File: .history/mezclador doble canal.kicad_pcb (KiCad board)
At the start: 2 copper layers, 166 x 100.5 mm, 17 parts, among them J1 Conn_Coaxial, J2 Conn_Coaxial, J3 Conn_Coaxial, U1 NE5532

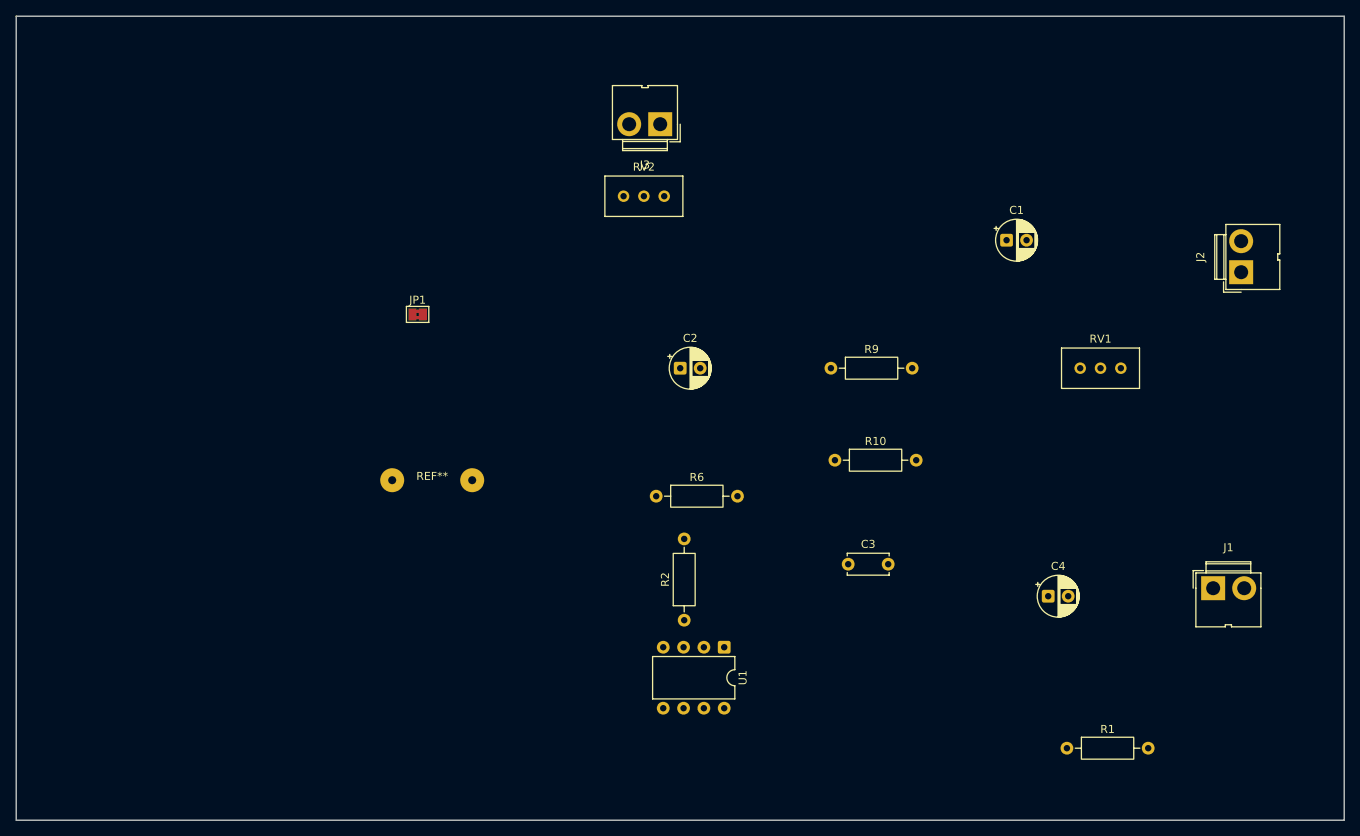
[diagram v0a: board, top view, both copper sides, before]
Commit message: completè el canal L
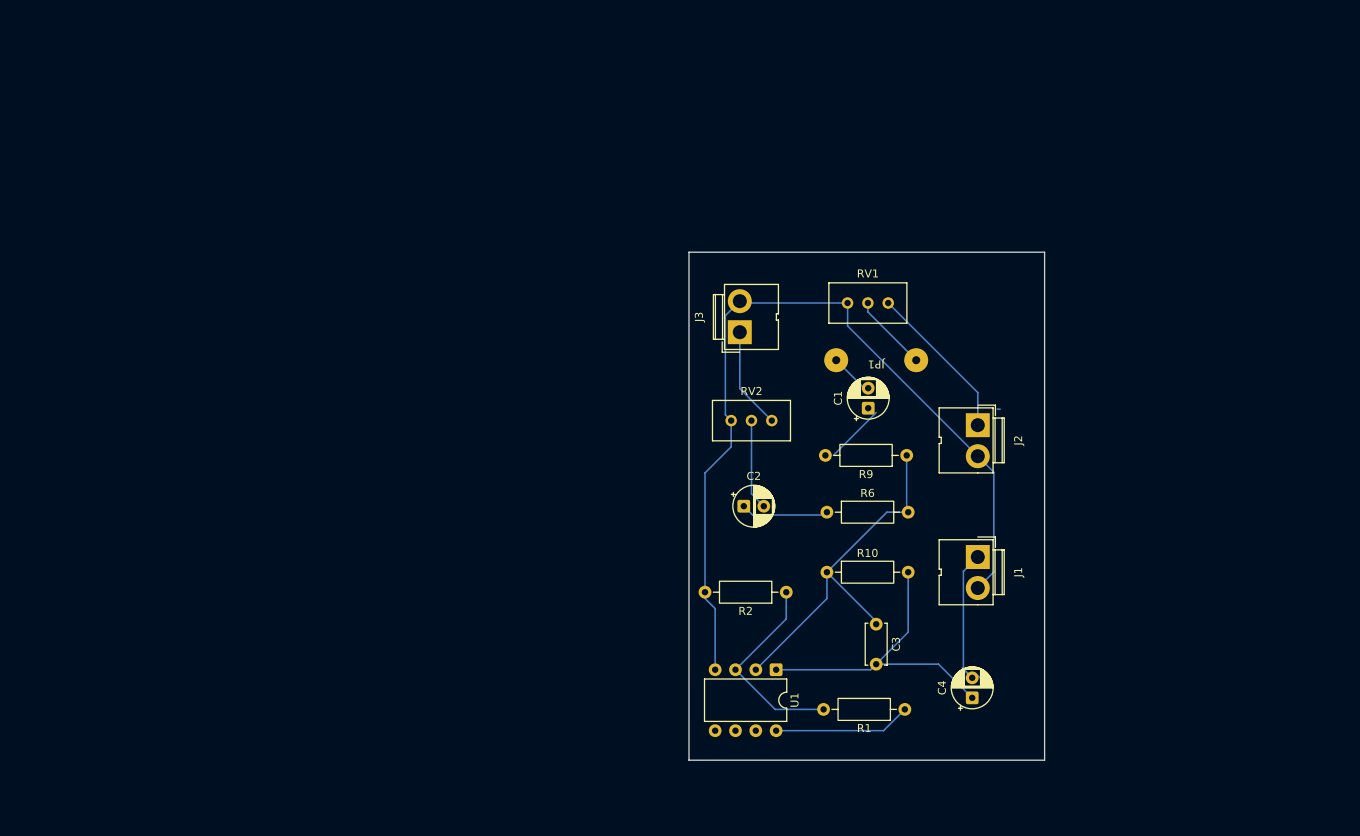
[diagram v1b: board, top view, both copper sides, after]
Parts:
- removed REF**: Jumper_Wire_10mm, personal:Jumper_Wire_10mm
- JP1: value Jumper_2_Bridged -> Jumper_2_Open; footprint Jumper:SolderJumper-2_P1.3mm_Bridged2Bar_Pad1.0x1.5mm -> personal:Jumper_Wire_10mm
- moved JP1 57.6 mm to (125.0, 77.0), turned to 180 degrees
- moved J2 38.1 mm to (137.7, 85.1), turned to -90 degrees
- moved RV2 31.1 mm to (112.0, 84.5)
- moved RV1 30.2 mm to (126.5, 69.8)
- moved J1 29.7 mm to (137.7, 101.6), turned to -90 degrees
- moved J3 27.8 mm to (108.0, 73.5), turned to 90 degrees
- moved C1 27.2 mm to (124.0, 83.0), turned to 90 degrees
- moved R6 21.4 mm to (118.8, 96.0)
- moved R1 20.8 mm to (128.6, 120.7), turned to 180 degrees
- moved C2 19.0 mm to (108.5, 95.2)
- moved C4 15.9 mm to (137.0, 119.2), turned to 90 degrees
- moved R9 14.4 mm to (128.8, 88.9), turned to 180 degrees
- moved R10 14.0 mm to (118.8, 103.5)
- moved R2 13.2 mm to (113.8, 106.0), turned to 180 degrees
- moved C3 8.28 mm to (125.0, 110.0), turned to -90 degrees
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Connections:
- C1 pad 2: Net-(C1-Pad2) -> Net-(JP1-B)
- JP1 pad 1: unconnected-(JP1-A-Pad1) -> Net-(JP1-A)
- JP1 pad 2: unconnected-(JP1-B-Pad2) -> Net-(JP1-B)
- RV1 pad 2: Net-(C1-Pad2) -> Net-(JP1-A)
- U1 pad 4: unconnected-(U1C-V--Pad4) -> GND
- U1 pad 8: unconnected-(U1C-V+-Pad8) -> VCC
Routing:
- net GND: track 0.00 -> 106.8 mm
- net Net-(U1A--): track 0.00 -> 45.9 mm
- net Net-(C3-Pad2): track 0.00 -> 39.7 mm
- net Net-(U1A-+): track 0.00 -> 25.4 mm
- net Net-(J2-In): track 0.00 -> 20.3 mm
- net Net-(J1-In): track 0.00 -> 18.4 mm
- net VCC: track 0.00 -> 17.2 mm
- net Net-(J3-In): track 0.00 -> 12.7 mm
- net Net-(C2-Pad2): track 0.00 -> 11.3 mm
- net Net-(C2-Pad1): track 0.00 -> 11.0 mm
- net Net-(JP1-A): track 0.00 -> 9.65 mm
- net Net-(C1-Pad1): track 0.00 -> 8.12 mm
- net Net-(JP1-B): track 0.00 -> 5.45 mm
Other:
- board size 166 x 100.5 mm -> 44.5 x 63.5 mm
